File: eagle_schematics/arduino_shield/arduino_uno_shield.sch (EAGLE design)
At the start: 20 parts

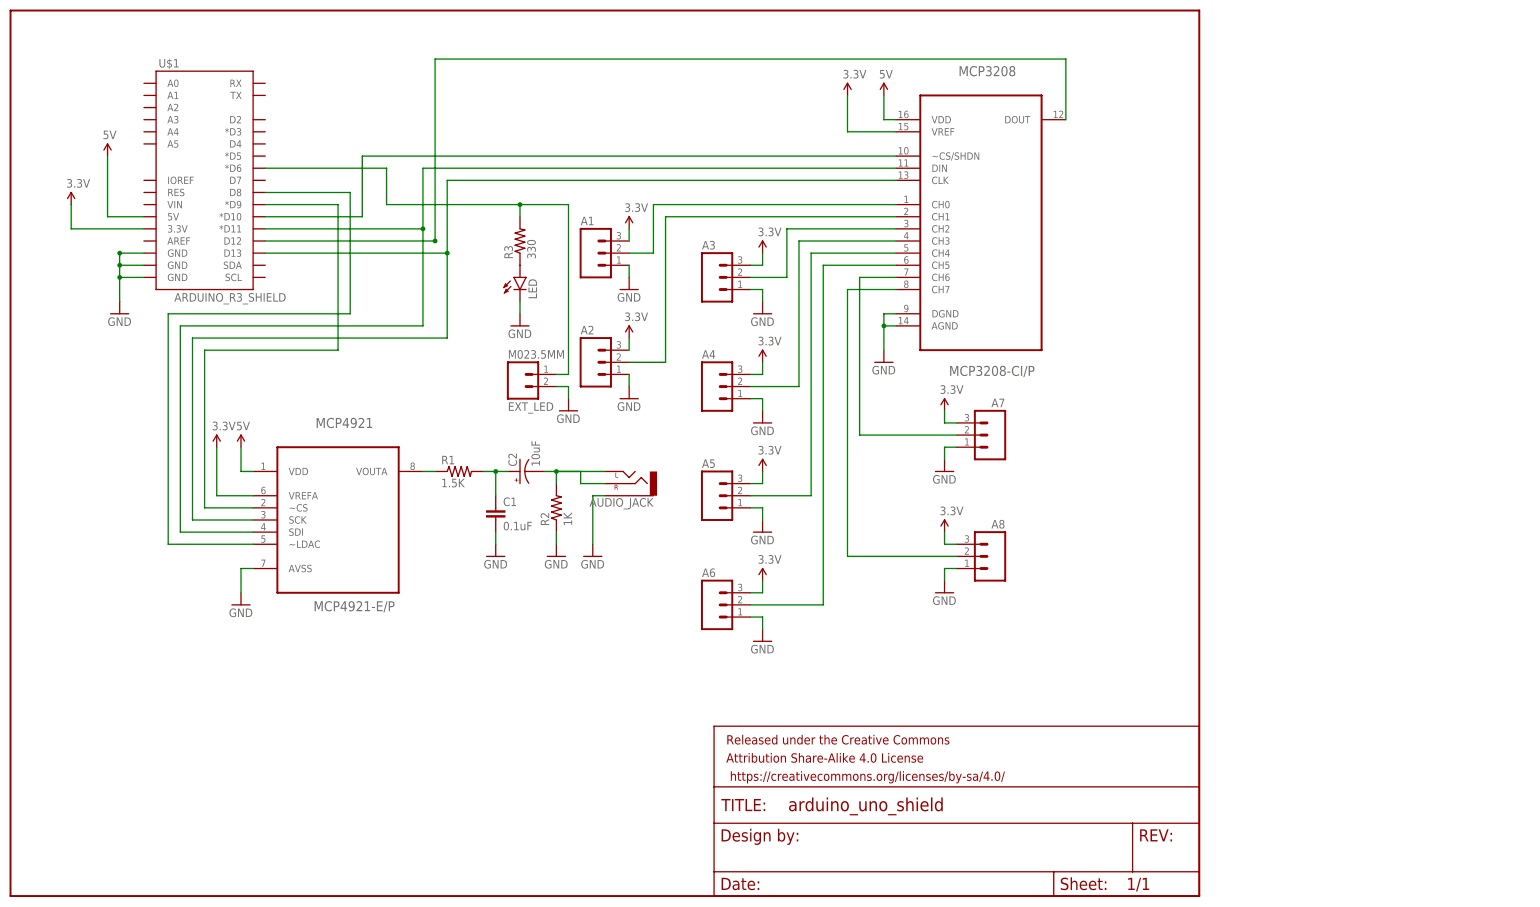
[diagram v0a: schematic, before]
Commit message: save
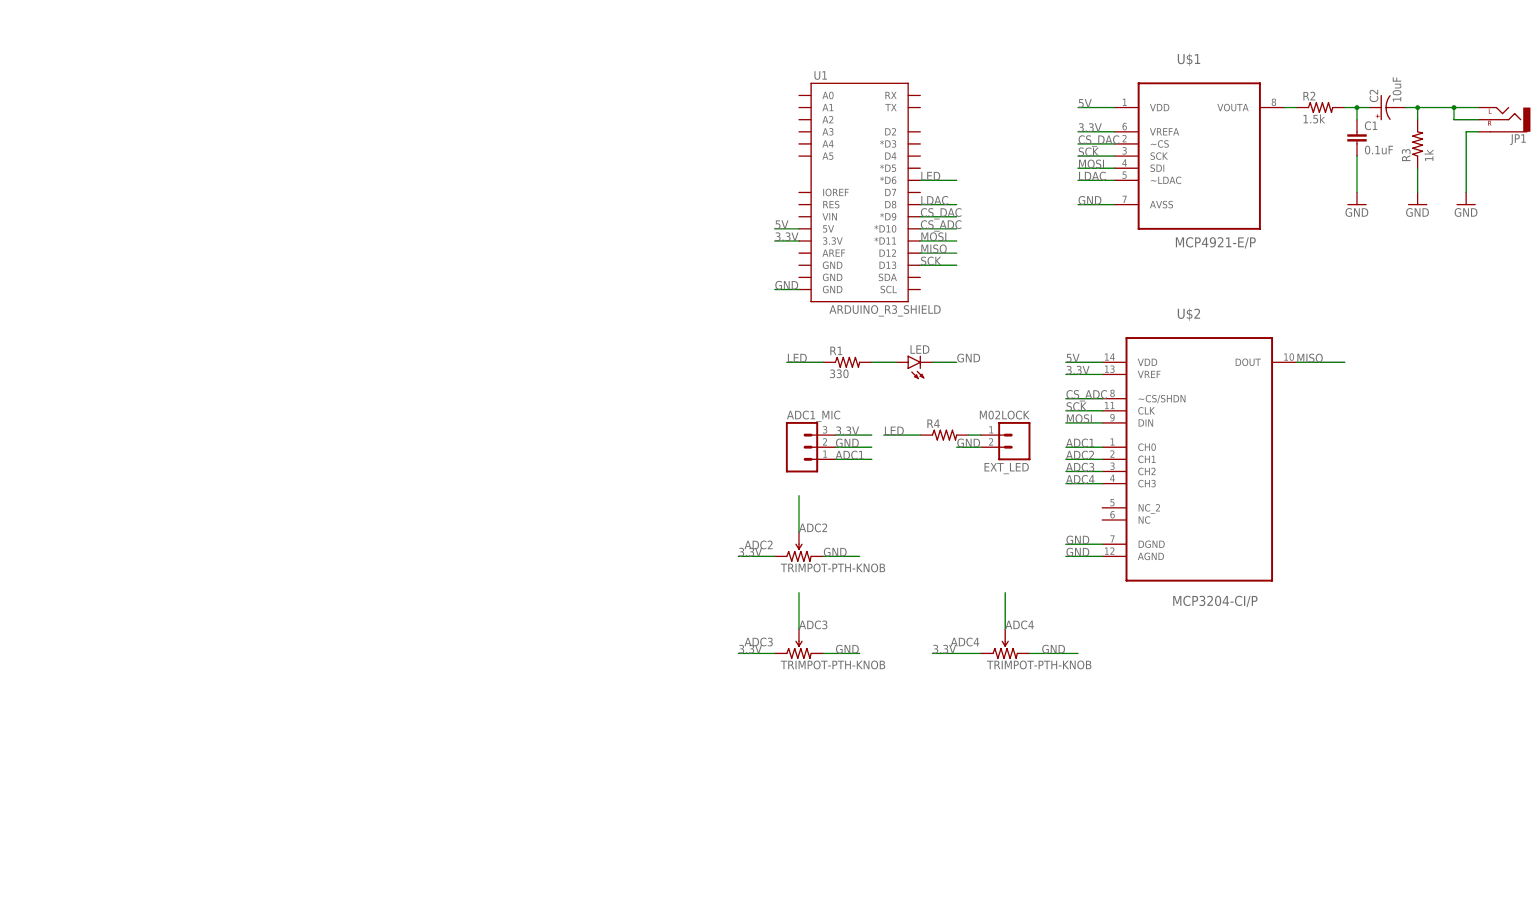
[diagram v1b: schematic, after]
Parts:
- removed A1, A2, A3, A4, A5, A6, A7, A8: (no value), SparkFun-Connectors:M03PTH
- removed AUDIO_JACK: (no value), SparkFun-Connectors:AUDIO-JACKPTH
- removed FRAME3: FRAME-LETTER, SparkFun-Aesthetics:FRAME-LETTER
- removed MCP3208: MCP3208-CI/P, Microchip_By_element14_Batch_1:MCP3208-CI/P
- removed MCP4921: MCP4921-E/P, Microchip_By_element14_Batch_1:MCP4921-E/P
- added ADC1_MIC: (no value), SparkFun-Connectors:M03LOCK
- added ADC2, ADC3, ADC4: TRIMPOT-PTH-KNOB, SparkFun-Electromechanical:TRIMPOT-PTH-KNOB
- added JP1: (no value), SparkFun-Connectors:AUDIO-JACKPTH
- added R4: (no value), SparkFun-Resistors:1KOHM-1/4W-5%(PTH)
- added U$2: MCP3204-CI/P, Microchip_By_element14_Batch_1:MCP3204-CI/P
- added U1: ARDUINO_R3_SHIELD, SparkFun-Boards:ARDUINO_R3_SHIELD
- C1: device SparkFun-Passives:CAPPTH -> SparkFun-Capacitors:CAPPTH1
- C2: device SparkFun-Passives:CAP_POLPTH2 -> SparkFun-Capacitors:CAP_POLPTH2
- EXT_LED: value M023.5MM -> M02LOCK; device SparkFun-Connectors:M023.5MM -> SparkFun-Connectors:M02LOCK
- R1: value 1.5K -> 330; device SparkFun-Passives:RESISTORPTH-1/4W -> SparkFun-Resistors:1KOHM-1/4W-5%(PTH)
- R2: value 1K -> 1.5k; device SparkFun-Passives:RESISTORPTH-1/4W -> SparkFun-Resistors:1KOHM-1/4W-5%(PTH)
- R3: value 330 -> 1k; device SparkFun-Passives:RESISTORPTH-1/4W -> SparkFun-Resistors:1KOHM-1/4W-5%(PTH)
- U$1: value ARDUINO_R3_SHIELD -> MCP4921-E/P; device SparkFun-Boards:ARDUINO_R3_SHIELD -> Microchip_By_element14_Batch_1:MCP4921-E/P
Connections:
- removed net AUD: A1.2, MCP3208.CH0
- removed net N$10: LED.A, R3.1
- removed net N$11: MCP4921.~LDAC, U$1.D8
- removed net N$12: EXT_LED.1, R3.2, U$1.*D6
- removed net N$14: A3.2, MCP3208.CH2
- removed net N$15: A4.2, MCP3208.CH3
- removed net N$16: A6.2, MCP3208.CH5
- removed net N$17: A7.2, MCP3208.CH6
- removed net N$18: A8.2, MCP3208.CH7
- removed net N$8: C1.1, C2.+, R1.2
- removed net N$9: AUDIO_JACK.LEFT, AUDIO_JACK.RIGHT, C2.-, R2.2
- removed net SPI_CLK: MCP3208.CLK, MCP4921.SCK, U$1.D13
- removed net SPI_MISO: MCP3208.DOUT, U$1.D12
- removed net SPI_MOSI: MCP3208.DIN, MCP4921.SDI, U$1.*D11
- new net ADC1: ADC1_MIC.1, U$2.CH0
- new net ADC2: ADC2.WIPER, U$2.CH1
- new net ADC3: ADC3.WIPER, U$2.CH2
- new net ADC4: ADC4.WIPER, U$2.CH3
- new net LDAC: U$1.~LDAC, U1.D8
- new net LED: R1.1, R4.1, U1.*D6
- new net MISO: U$2.DOUT, U1.D12
- new net MOSI: U$1.SDI, U$2.DIN, U1.*D11
- new net N$4: C2.-, JP1.LEFT, JP1.RIGHT, R3.2
- new net N$5: EXT_LED.1, R4.2
- new net SCK: U$1.SCK, U$2.CLK, U1.D13
- net 3.3V: now also ADC1_MIC.3, ADC2.CCW, ADC3.CCW, ADC4.CCW, U$1.VREFA, U$2.VREF, U1.3.3V; no longer A1.3, A2.3, A3.3, A4.3, A5.3, A6.3, A7.3, A8.3, MCP3208.VREF, MCP4921.VREFA, U$1.3.3V
- net 5V: now also U$1.VDD, U$2.VDD, U1.5V; no longer MCP3208.VDD, MCP4921.VDD, U$1.5V
- net CS_ADC: now also U$2.~CS/SHDN, U1.*D10; no longer MCP3208.~CS/SHDN, U$1.*D10
- net CS_DAC: now also U$1.~CS, U1.*D9; no longer MCP4921.~CS, U$1.*D9
- net GND: now also ADC1_MIC.2, ADC2.CW, ADC3.CW, ADC4.CW, JP1.SLEEVE, R3.1, U$1.AVSS, U$2.AGND, U$2.DGND, U1.GND@0; no longer A1.1, A2.1, A3.1, A4.1, A5.1, A6.1, A7.1, A8.1, AUDIO_JACK.SLEEVE, MCP3208.AGND, MCP3208.DGND, MCP4921.AVSS, R2.1, U$1.GND@0, U$1.GND@1, U$1.GND@2
- net N$1: now also LED.A, R1.2; no longer A5.2, MCP3208.CH4
- net N$2: now also R2.1, U$1.VOUTA; no longer A2.2, MCP3208.CH1
- net N$3: now also C1.1, C2.+, R2.2; no longer MCP4921.VOUTA, R1.1
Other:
- moved on the sheet: C1, C2, EXT_LED, LED, R1, R2, R3

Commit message: change resistors from AXIAL-0.3 to AXIAL-0.4
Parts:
- R1, R2, R3, R4: device SparkFun-Resistors:1KOHM-1/4W-5%(PTH) -> SparkFun-Resistors:RESISTORPTH-1/4W
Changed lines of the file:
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@@
 <part name="U$1" library="Microchip_By_element14_Batch_1" deviceset="MCP4921-E/P" device=""/>
 <part name="U$2" library="Microchip_By_element14_Batch_1" deviceset="MCP3204-CI/P" device=""/>
-<part name="R1" library="SparkFun-Resistors" deviceset="1KOHM-1/4W-5%(PTH)" device="" value="330"/>
-<part name="R2" library="SparkFun-Resistors" deviceset="1KOHM-1/4W-5%(PTH)" device="" value="1.5k"/>
-<part name="R3" library="SparkFun-Resistors" deviceset="1KOHM-1/4W-5%(PTH)" device="" value="1k"/>
+<part name="R1" library="SparkFun-Resistors" deviceset="RESISTOR" device="PTH-1/4W" value="330"/>
+<part name="R2" library="SparkFun-Resistors" deviceset="RESISTOR" device="PTH-1/4W" value="1.5k"/>
+<part name="R3" library="SparkFun-Resistors" deviceset="RESISTOR" device="PTH-1/4W" value="1k"/>
 <part name="LED" library="SparkFun-LED" deviceset="LED" device="5MM"/>
 <part name="C1" library="SparkFun-Capacitors" deviceset="CAP" device="PTH1" value="0.1uF"/>
@@
 <part name="ADC1_MIC" library="SparkFun-Connectors" deviceset="M03" device="LOCK"/>
 <part name="EXT_LED" library="SparkFun-Connectors" deviceset="M02" device="LOCK"/>
-<part name="R4" library="SparkFun-Resistors" deviceset="1KOHM-1/4W-5%(PTH)" device=""/>
+<part name="R4" library="SparkFun-Resistors" deviceset="RESISTOR" device="PTH-1/4W"/>
 <part name="ADC2" library="SparkFun-Electromechanical" deviceset="TRIMPOT" device="-PTH-KNOB"/>
 <part name="ADC3" library="SparkFun-Electromechanical" deviceset="TRIMPOT" device="-PTH-KNOB"/>
